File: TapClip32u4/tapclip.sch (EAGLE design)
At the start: 32 parts, among them X1 USBSMD, Y1 16MHz

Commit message: Keeping up with the Jones's
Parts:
- added C11, C12: (no value), SparkFun:CAP0603-CAP
- added R4, R5, R6: (no value), SparkFun:RESISTOR0603-RES
- added U$13, U$14, U$15, U$16, U$17, U$18: ALLIGATOR_CLIP, sdgj:ALLIGATOR_CLIP
- added U$19, U$22: LTC1391-MUX, sdgj:LTC1391-MUX
- added U$20: PGA112, sdgj:PGA112
- added U$21: ADG704-MUX, sdgj:ADG704-MUX
- U$2: value PGA116 -> ALLIGATOR_CLIP; device sdgj:PGA116 -> sdgj:ALLIGATOR_CLIP
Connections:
- removed net CS: U$2.CS
- removed net EN: U$2.EN
- removed net N$15: U$1.PD7(OC4D/ADC10/T0)
- new net CS1: U$19.CS, U$22.CS
- new net CS2: U$20.CS
- new net D: R6.1, U$19.D, U$20.CH1, U$21.S4, U$22.D
- new net MA0: U$1.PD7(OC4D/ADC10/T0), U$21.A0
- new net MA1: U$1.PD6(T1/ADC9/!OC4D), U$21.A1
- new net MDOUT: U$19.DOUT, U$22.DIN
- new net MS1: R4.2, U$21.S1
- new net MS2: R4.1, R5.2, U$21.S3
- new net MS3: R5.1, R6.2, U$21.S2
- new net N$22: C2.1, U$19.V+
- new net N$30: U$20.CH0
- new net N$36: U$21.EN
- new net PB4: U$21.D
- new net S10: U$2.SNS, U$22.S2
- new net S11: U$13.SNS, U$22.S3
- new net S12: U$14.SNS, U$22.S4
- new net S13: U$15.SNS, U$22.S5
- new net S14: U$16.SNS, U$22.S6
- new net S15: U$17.SNS, U$22.S7
- new net S16: U$18.SNS
- new net SCLK: U$1.PB1(SCK), U$19.CLK, U$20.SCLK, U$22.CLK
- net GND: now also C11.2, C12.2, U$19.GND, U$19.V-, U$20.GND, U$20.VREF, U$21.GND, U$22.GND, U$22.V-; no longer U$2.GND
- net MISO: no longer U$2.DOUT
- net MOSI: now also U$19.DIN, U$20.DIO; no longer U$2.DIN
- net N$14: now also C12.1, U$22.V+; no longer U$1.PD6(T1/ADC9/!OC4D)
- net S0: now also U$19.S0; no longer U$2.CH0
- net S1: now also U$19.S1; no longer U$2.CH1
- net S2: now also U$19.S2; no longer U$2.CH2
- net S3: now also U$19.S3; no longer U$2.CH3
- net S4: now also U$19.S4; no longer U$2.CH4
- net S5: now also U$19.S5; no longer U$2.CH5
- net S6: now also U$19.S6; no longer U$2.CH6
- net S7: now also U$19.S7; no longer U$2.CH7
- net S8: now also U$22.S0; no longer U$2.CH8
- net S9: now also U$22.S1; no longer U$2.CH9
- net SCK: no longer U$1.PB1(SCK), U$2.SCLK
- net VCC: now also C11.1, U$20.AVDD, U$20.DVDD, U$21.VDD; no longer C2.1, U$2.AVDD, U$2.DVDD
- net VOUT: now also U$20.VOUT; no longer U$2.VOUT, U$2.VREF
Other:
- note removed: "these are regular IO"
- moved on the sheet: C10, C2

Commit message: Much has taken place here. Be still. Breath. Prepare yonder Gerbers.
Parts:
- removed RN1: 10K, resistor-dil:4R-NCAY16
- removed U$10, U$11, U$13, U$14, U$15, U$16, U$17, U$18, U$3, U$4, U$5, U$6, U$8, U$9: ALLIGATOR_CLIP, sdgj:ALLIGATOR_CLIP
- removed U$22: LTC1391-MUX, sdgj:LTC1391-MUX
- added JP1: (no value), adafruit:PINHD-1X6CB
- added LED3, LED4, LED5, LED6, LED7, LED8: GREEN, SparkFun:LED0603
- added R20, R21, R22: 330, SparkFun-Passives:RESISTOR0402-RES
- added R8: (no value), SparkFun:RESISTOR0603-RES
- added S1, S2, S4, S5, S6, S7: ALLIGATOR_CLIP, sdgj:ALLIGATOR_CLIP
- added SJ1, SJ2: SOLDERJUMPERTRACE, SparkFun:SOLDERJUMPERTRACE
- added SJ3, SJ4: SOLDERJUMPERNO, SparkFun:SOLDERJUMPERNO
- C10, C11, C12, C2, C5: value (none) -> .1uF
- LED1: device SparkFun:LED1206 -> SparkFun:LED0603
- R3: value (none) -> 300
- U$2: value ALLIGATOR_CLIP -> LTC1391-MUX; device sdgj:ALLIGATOR_CLIP -> sdgj:LTC1391-MUX
- renumbered U$12 to S3, U$7 to S8
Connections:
- removed net N$14: C12.1, U$22.V+
- removed net N$16: U$1.PC6(OC3A/!OC4A)
- removed net N$17: U$1.PC7(ICP3/CLK0/OC4A)
- removed net N$20: U$1.PB5(OC1A/ADC12/!OC4B)
- removed net N$21: U$1.PB4(ADC11)
- removed net N$3: U$1.PE2(!HWB)
- removed net N$4: U$1.PE6(INT.6/AIN0)
- removed net S10: U$2.SNS, U$22.S2
- removed net S11: U$13.SNS, U$22.S3
- removed net S12: U$14.SNS, U$22.S4
- removed net S13: U$15.SNS, U$22.S5
- removed net S14: U$16.SNS, U$22.S6
- removed net S15: U$17.SNS, U$22.S7
- removed net S16: U$18.SNS
- removed net S8: U$10.SNS, U$22.S0
- removed net S9: U$11.SNS, U$22.S1
- removed net SCK: ICSP.3
- new net J0: JP1.1, U$1.PF4(ADC4/TCK)
- new net J1: JP1.2, U$1.PE2(!HWB)
- new net J2: JP1.3, U$1.PE6(INT.6/AIN0)
- new net J3: JP1.4, U$1.PC6(OC3A/!OC4A)
- new net J4: JP1.5, U$1.PC7(ICP3/CLK0/OC4A)
- new net J5: JP1.6, U$1.PB7(OC0A/OC1C/RTS)
- new net LED0: R20.1, U$1.PB4(ADC11)
- new net LED1: R21.1, U$1.PB6(OC1B/OC4B/ADC13)
- new net LED2: R22.1, U$1.PB5(OC1A/ADC12/!OC4B)
- new net N$15: S1.SNS, SJ2.2, SJ3.2
- new net N$24: LED5.A, LED6.C, LED7.A, LED8.C, R21.2
- new net N$25: LED3.A, LED4.C, LED7.C, LED8.A, R20.2
- new net N$26: LED3.C, LED4.A, LED5.C, LED6.A, R22.2
- new net VOUT1: U$1.PF1(ADC1), U$2.D
- net CS1: now also U$2.CS; no longer U$22.CS
- net D: no longer U$22.D
- net GND: now also SJ4.1, U$2.GND, U$2.V-; no longer U$22.GND, U$22.V-
- net MA0: now also U$1.PF6(ADC6/TDO); no longer U$1.PD7(OC4D/ADC10/T0)
- net MA1: now also U$1.PF5(ADC5/TMS); no longer U$1.PD6(T1/ADC9/!OC4D)
- net MDOUT: now also U$2.DIN; no longer U$22.DIN
- net N$18: now also U$1.PF7(ADC7(TDI); no longer U$1.PB7(OC0A/OC1C/RTS)
- net N$19: now also S2.SNS, SJ1.2, SJ4.2; no longer U$1.PB6(OC1B/OC4B/ADC13)
- net RESET: now also R8.1; no longer RN1D.1
- net S0: now also S8.SNS, U$2.S0; no longer S3.SNS
- net S1: now also S7.SNS, U$2.S1; no longer U$3.SNS
- net S2: now also S6.SNS, U$2.S2; no longer U$4.SNS
- net S3: now also S5.SNS, U$2.S3; no longer U$5.SNS
- net S4: now also S4.SNS, U$2.S4; no longer U$6.SNS
- net S5: now also S3.SNS, U$2.S5; no longer S8.SNS
- net S6: now also SJ1.1, U$2.S6; no longer U$8.SNS
- net S7: now also SJ2.1, U$2.S7; no longer U$9.SNS
- net SCLK: now also ICSP.3, U$2.CLK; no longer U$22.CLK
- net VCC: now also C12.1, R8.2, SJ3.1, U$2.V+; no longer RN1D.2
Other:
- moved on the sheet: C12

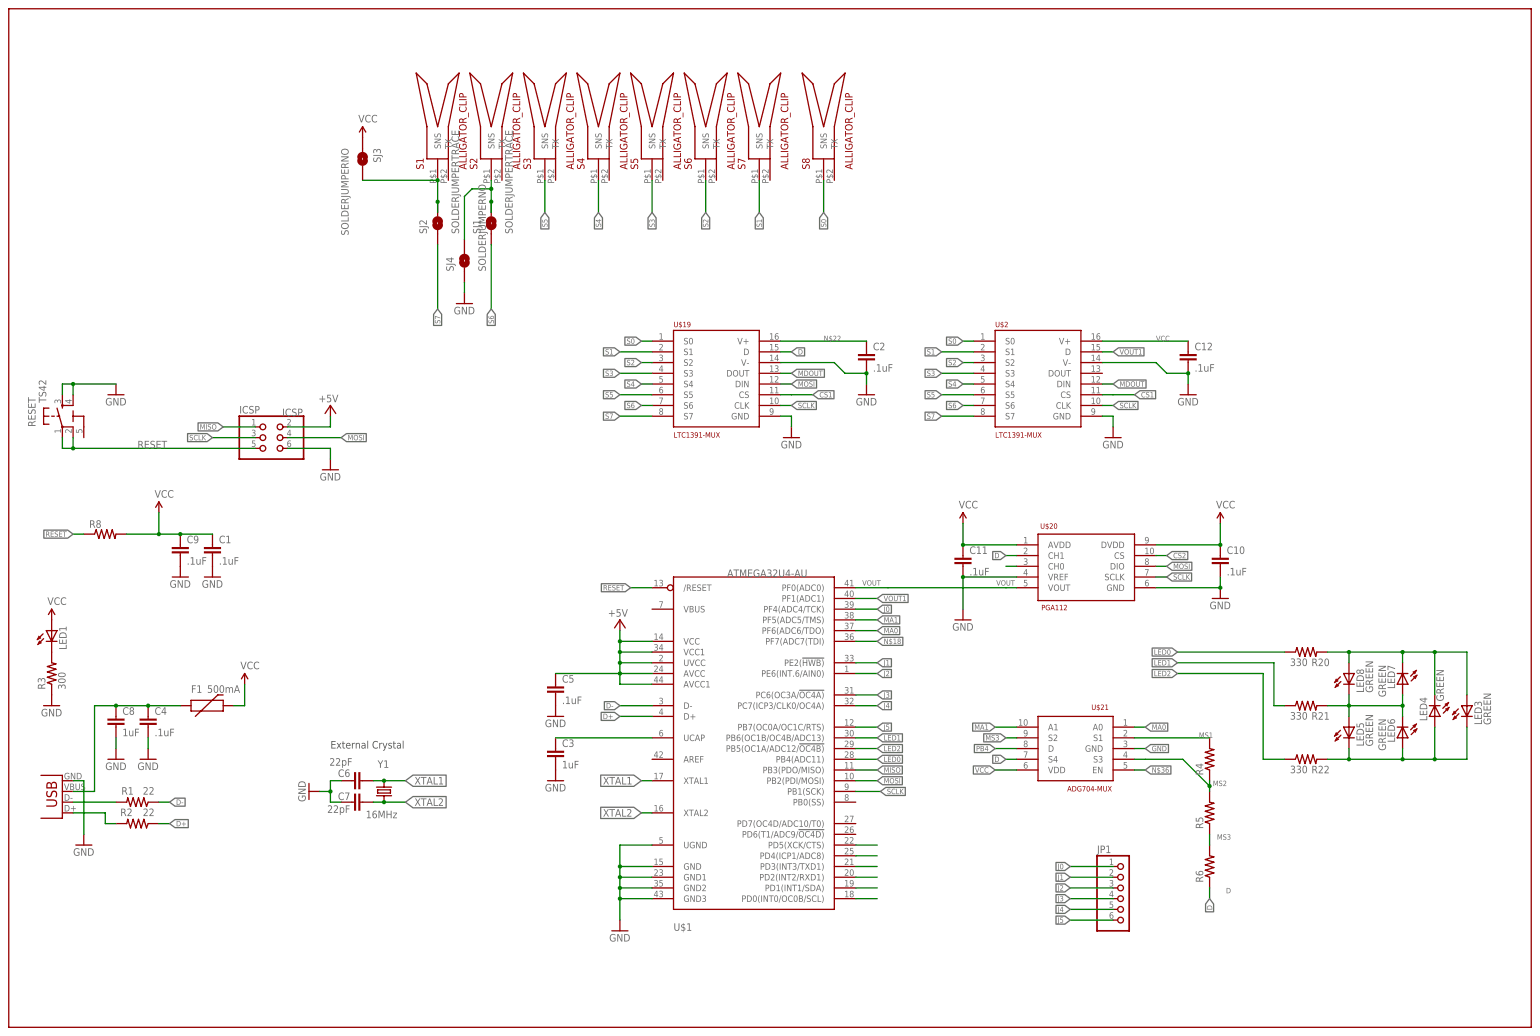
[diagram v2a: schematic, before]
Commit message: And we've entered the rodeo.
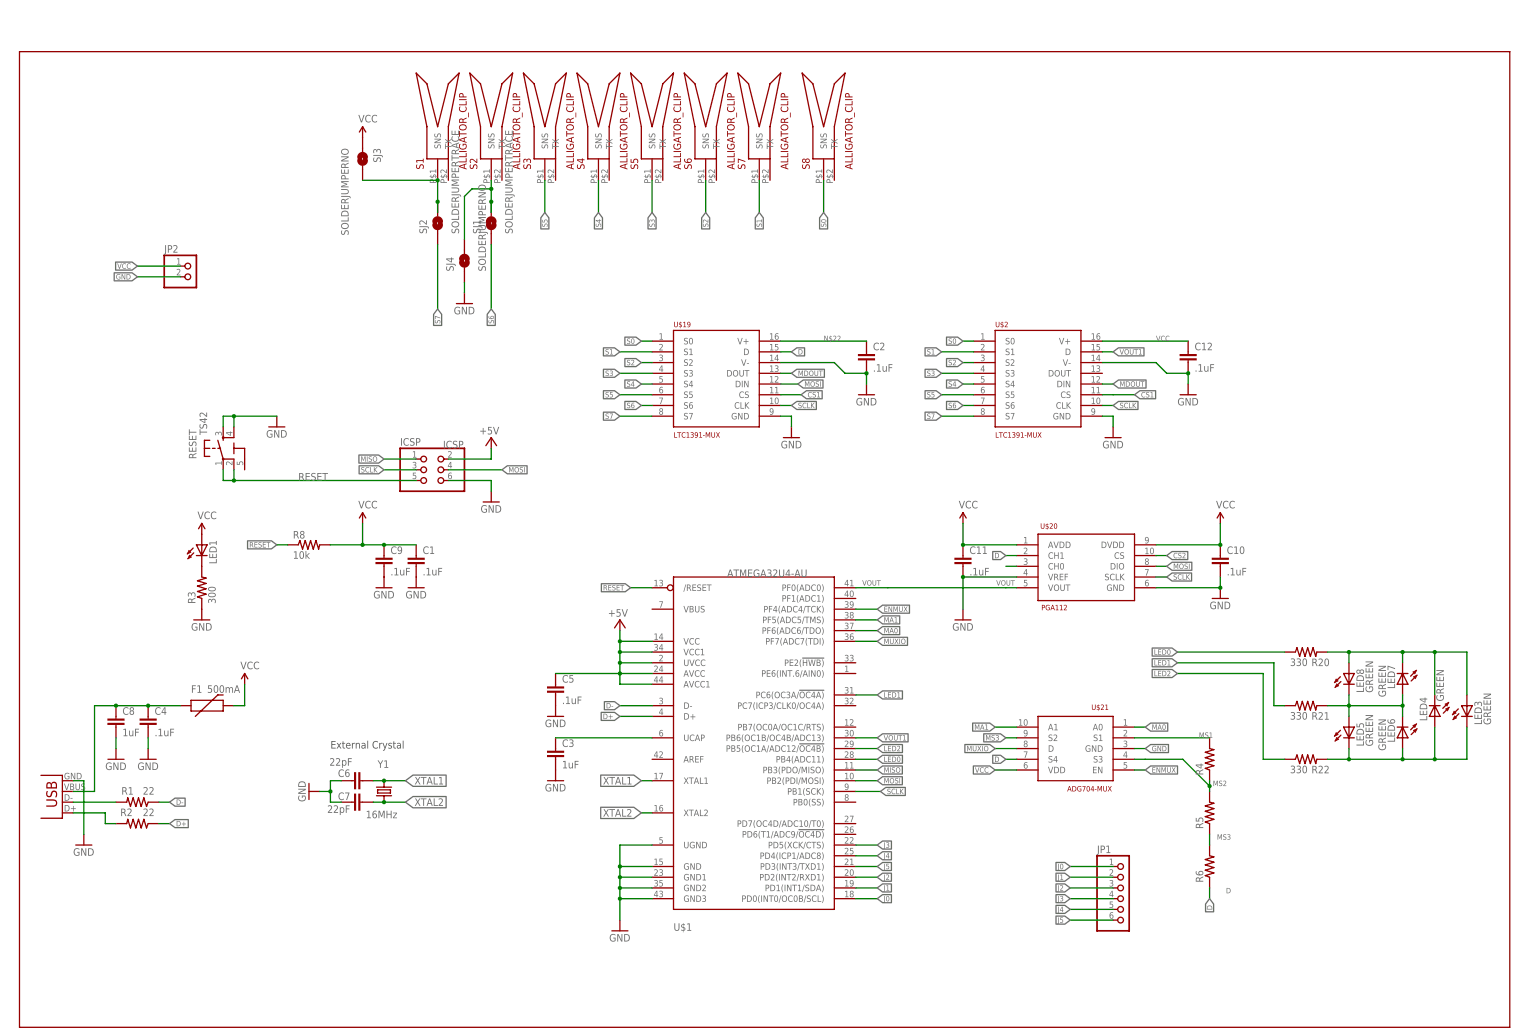
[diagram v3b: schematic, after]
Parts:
- added JP2: (no value), pinhead:PINHD-1X2
- R8: value (none) -> 10k
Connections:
- removed net N$10: U$1.PD2(INT2/RXD1)
- removed net N$11: U$1.PD3(INT3/TXD1)
- removed net N$12: U$1.PD4(ICP1/ADC8)
- removed net N$13: U$1.PD5(XCK/CTS)
- removed net N$18: U$1.PF7(ADC7(TDI)
- removed net N$36: U$21.EN
- removed net N$7: U$1.PD0(INT0/OC0B/SCL)
- removed net N$9: U$1.PD1(INT1/SDA)
- removed net PB4: U$21.D
- new net ENMUX: U$1.PF4(ADC4/TCK), U$21.EN
- new net MUXIO: U$1.PF7(ADC7(TDI), U$21.D
- net GND: now also JP2.2
- net J0: now also U$1.PD0(INT0/OC0B/SCL); no longer U$1.PF4(ADC4/TCK)
- net J1: now also U$1.PD1(INT1/SDA); no longer U$1.PE2(!HWB)
- net J2: now also U$1.PD2(INT2/RXD1); no longer U$1.PE6(INT.6/AIN0)
- net J3: now also U$1.PD5(XCK/CTS); no longer U$1.PC6(OC3A/!OC4A)
- net J4: now also U$1.PD4(ICP1/ADC8); no longer U$1.PC7(ICP3/CLK0/OC4A)
- net J5: now also U$1.PD3(INT3/TXD1); no longer U$1.PB7(OC0A/OC1C/RTS)
- net LED1: now also U$1.PC6(OC3A/!OC4A); no longer U$1.PB6(OC1B/OC4B/ADC13)
- net VCC: now also JP2.1
- net VOUT1: now also U$1.PB6(OC1B/OC4B/ADC13); no longer U$1.PF1(ADC1)
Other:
- moved on the sheet: C1, C9, ICSP, LED1, R3, R8, RESET
